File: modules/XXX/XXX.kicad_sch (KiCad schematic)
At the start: 25 parts, among them J1 CardConnector, SW1 SW_SPDT_MSM, SW2 SW_SPDT_MSM, SW3 SW_SPDT_MSM, SW4 SW_SPDT_MSM, SW5 SW_SPDT_MSM, SW6 SW_SPDT_MSM, SW7 SW_SPDT_MSM, SW8 SW_SPDT_MSM

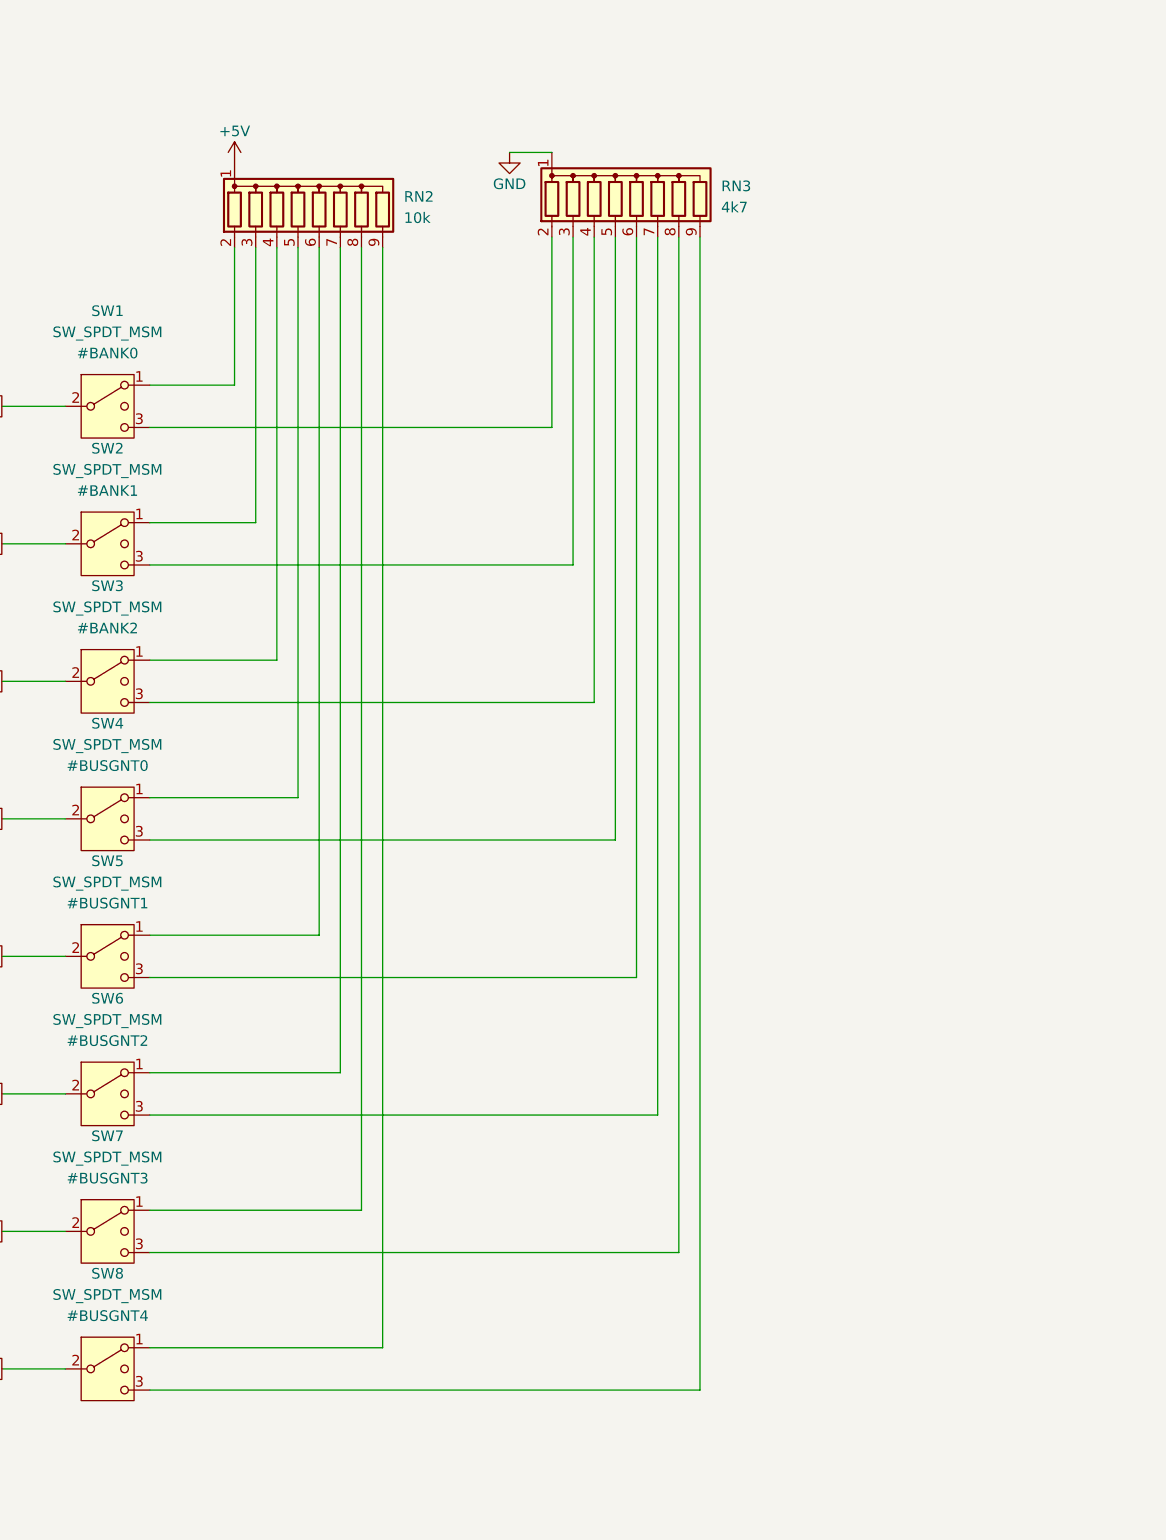
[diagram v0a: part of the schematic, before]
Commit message: work on RAM and bus terminator
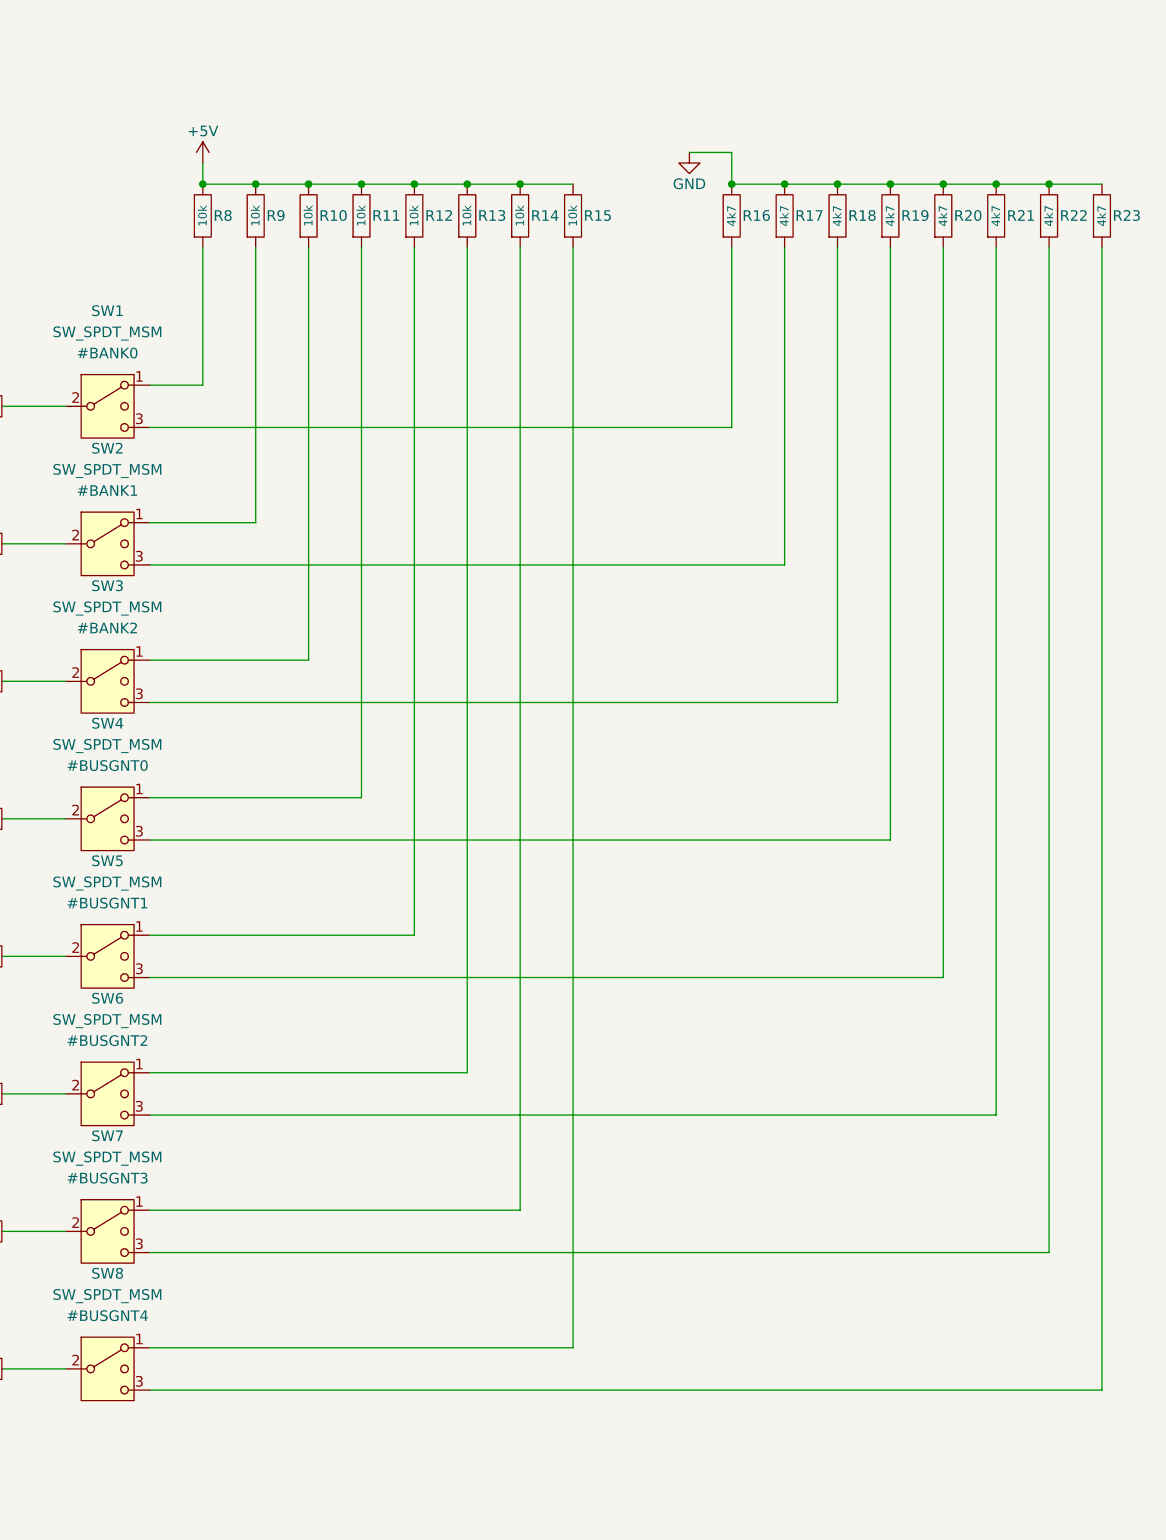
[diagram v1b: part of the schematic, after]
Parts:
- removed RN2: 10k, Resistor_THT:R_Array_SIP9, symbol Device:R_Network08
- removed RN3: 4k7, Resistor_THT:R_Array_SIP9, symbol Device:R_Network08
- added R10, R11, R12, R13, R14, R15, R8, R9: 10k, IMNOTWOPR:R_Axial_DIN0207_P400mil, symbol IMNOTWOPR:R_Vertical
- added R16, R17, R18, R19, R20, R21, R22, R23: 4k7, IMNOTWOPR:R_Axial_DIN0207_P400mil, symbol IMNOTWOPR:R_Vertical
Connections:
- net +5V: now also R10.2, R11.2, R12.2, R13.2, R14.2, R15.2, R8.2, R9.2
- net GND: now also R16.2, R17.2, R18.2, R19.2, R20.2, R21.2, R22.2, R23.2
- net at SW2.1: now also R9.1
- net at SW2.3 (4): now also R17.1
- net at SW6.1: now also R13.1
- net at SW6.3 (4): now also R21.1
- net at SW1.1: now also R8.1
- net at SW1.3 (4): now also R16.1
- net at SW4.1: now also R11.1
- net at SW4.3 (4): now also R19.1
- net at SW3.1: now also R10.1
- net at SW5.1: now also R12.1
- net at SW7.1: now also R14.1
- net at SW8.1: now also R15.1
- net at SW7.3 (4): now also R22.1
- net at SW5.3 (4): now also R20.1
- net at SW3.3 (4): now also R18.1
- net at SW8.3 (4): now also R23.1
